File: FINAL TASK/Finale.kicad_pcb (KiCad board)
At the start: 2 copper layers, 58.2 x 41.1 mm, 31 parts, among them J1 Conn_01x04_Pin, J2 Conn_01x04_Pin, P1 USB_C_Plug, SW1 RESET, SW2 SW_SPDT, U1 STM32F103C8T6, U2 AS5048B, U3 AS5048B, U4 AS5048B, U5 AS5048B, U6 AMS1117-3.3, Y1 16MHz

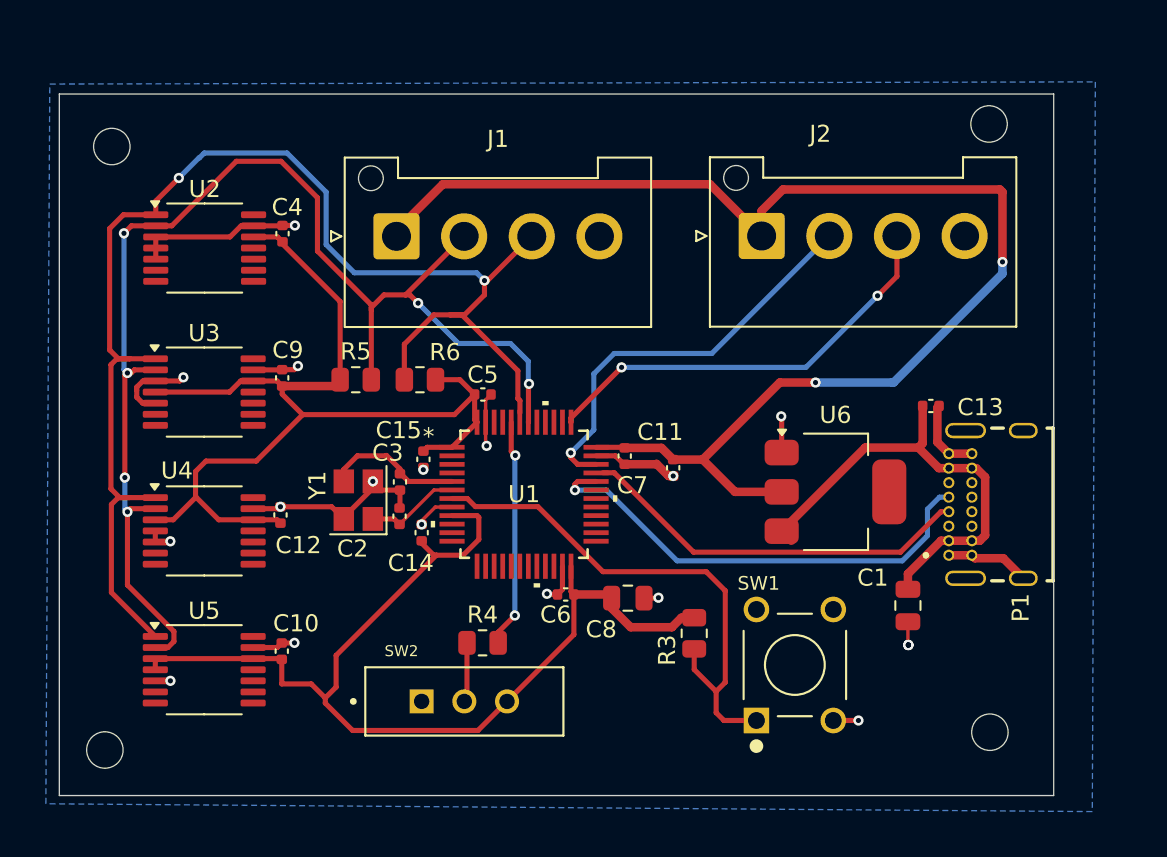
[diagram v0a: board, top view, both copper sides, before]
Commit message: Done
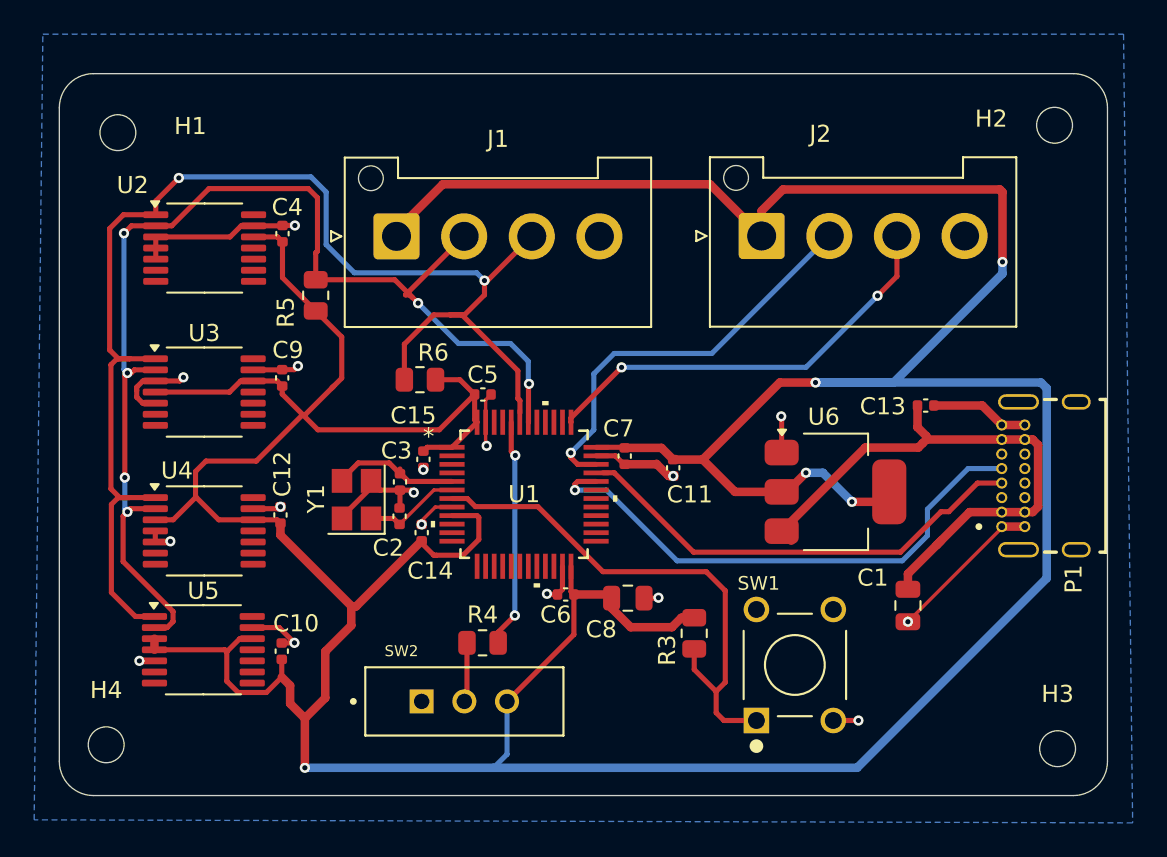
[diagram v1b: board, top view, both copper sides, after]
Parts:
- added H1: MountingHole, MountingHole:MountingHole_2.1mm, F.Cu at (138.0, 72.2)
- added H2: MountingHole, MountingHole:MountingHole_2.1mm, F.Cu at (192.8, 71.7)
- added H3: MountingHole, MountingHole:MountingHole_2.1mm, F.Cu at (193.0, 108.2)
- added H4: MountingHole, MountingHole:MountingHole_2.1mm, F.Cu at (137.3, 108.0)
- moved R5 5.47 mm to (149.6, 81.7), turned to 90 degrees
- moved P1 3.52 mm to (194.1, 92.3)
- moved U5 1.17 mm to (143.0, 102.4)
- moved C13 0.30 mm to (185.3, 88.1)
- moved Y1 0.11 mm to (151.9, 93.6)
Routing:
- net +3.3V: track 201.1 -> 289.8 mm, vias 2 -> 5
- net VBUS: track 27.8 -> 34.5 mm
- net /I2C_SCL: track 75.5 -> 69.7 mm
- net /DP: track 23.2 -> 27.0 mm
- net /DM: track 27.7 -> 31.5 mm
- net GND: track 62.3 -> 64.4 mm, vias 19 -> 17
- net /I2C_SDA: track 80.9 -> 79.3 mm
- net /OSC_IN: track 8.17 -> 7.67 mm
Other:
- board size 58.2 x 41.1 mm -> 61.4 x 42.3 mm
- board text added: "U2"
